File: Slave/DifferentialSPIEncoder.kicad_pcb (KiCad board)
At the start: 2 copper layers, 35.6 x 21.6 mm, 26 parts, among them J1 debug, J2 8P8C_Shielded, U1 TLV71333PDBV, U2 AS5048A, U3 MAX485E, U4 MAX485E, U5 MAX485E

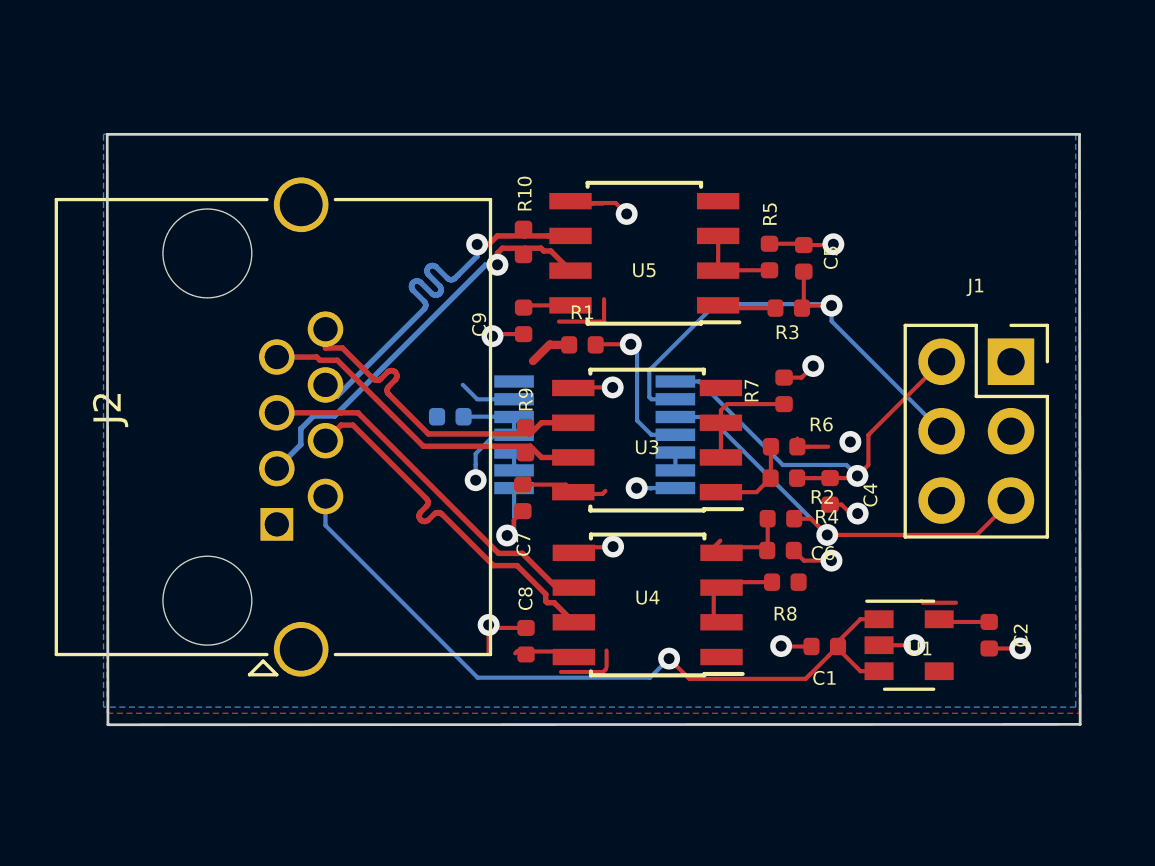
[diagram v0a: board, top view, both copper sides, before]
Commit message: next version
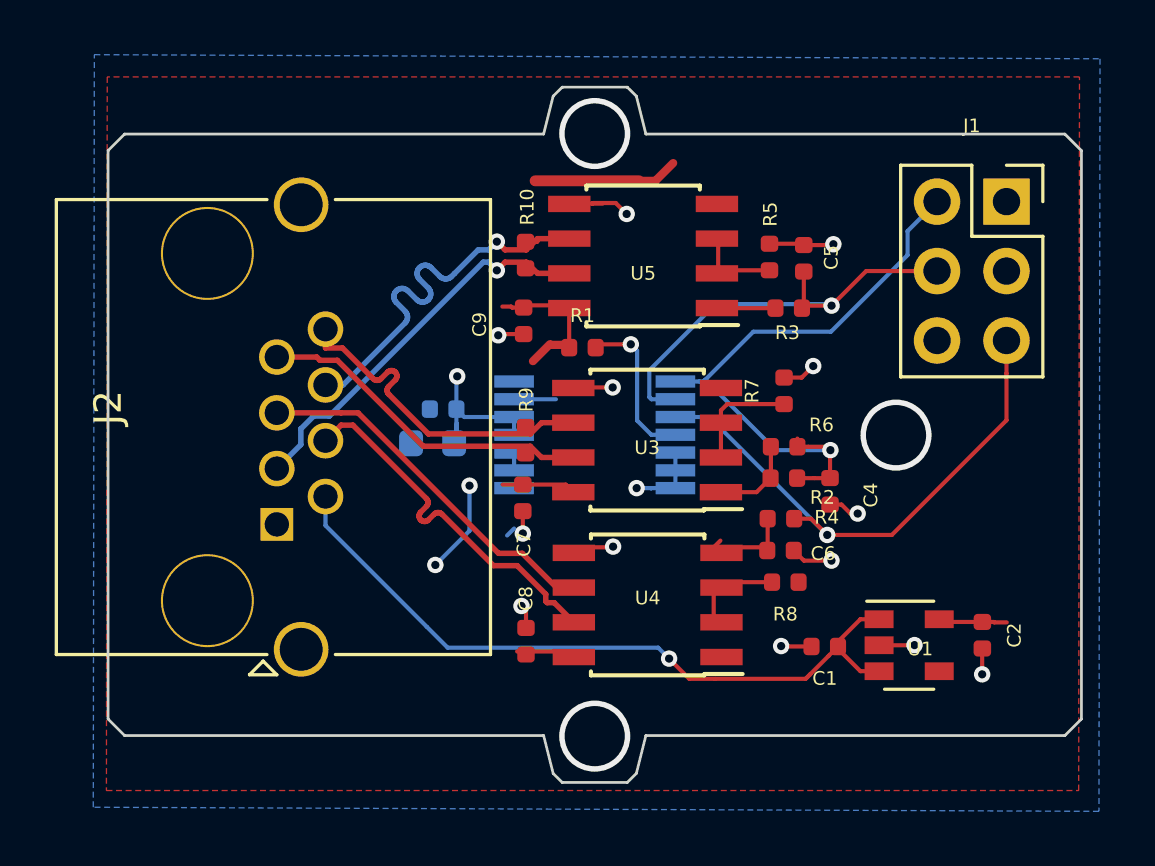
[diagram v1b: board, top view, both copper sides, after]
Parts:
- added C10: 10uF, Capacitor_SMD:C_0603_1608Metric, B.Cu at (107.2, 66.3)
- moved J1 5.86 mm to (128.1, 57.5)
- moved R10 0.49 mm to (110.5, 59.4)
- moved C3 0.38 mm to (107.5, 65.0)
- moved C2 0.25 mm to (127.3, 73.3)
- moved U5 0.11 mm to (114.8, 59.5)
- moved R1 0.10 mm to (112.6, 62.8)
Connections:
- J2 pad SH: GND -> Net-(J2-PadSH)
- R6 pad 1: +3V3 -> ~CSn
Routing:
- net +3V3: track 17.7 -> 27.5 mm, vias 2 -> 3
- net ~CSn: track 16.0 -> 22.3 mm
- net (no net): track 6.06 -> 0.00 mm, vias 0 -> 3
- net MISO: track 16.0 -> 20.0 mm
- net GND: track 27.3 -> 23.6 mm
- net CLK: track 18.4 -> 16.5 mm
- net /CLK_-: track 15.3 -> 14.6 mm
- net +5V: track 27.3 -> 26.7 mm
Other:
- board size 35.6 x 21.6 mm -> 35.6 x 25.4 mm
